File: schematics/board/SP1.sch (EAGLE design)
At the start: 12 parts

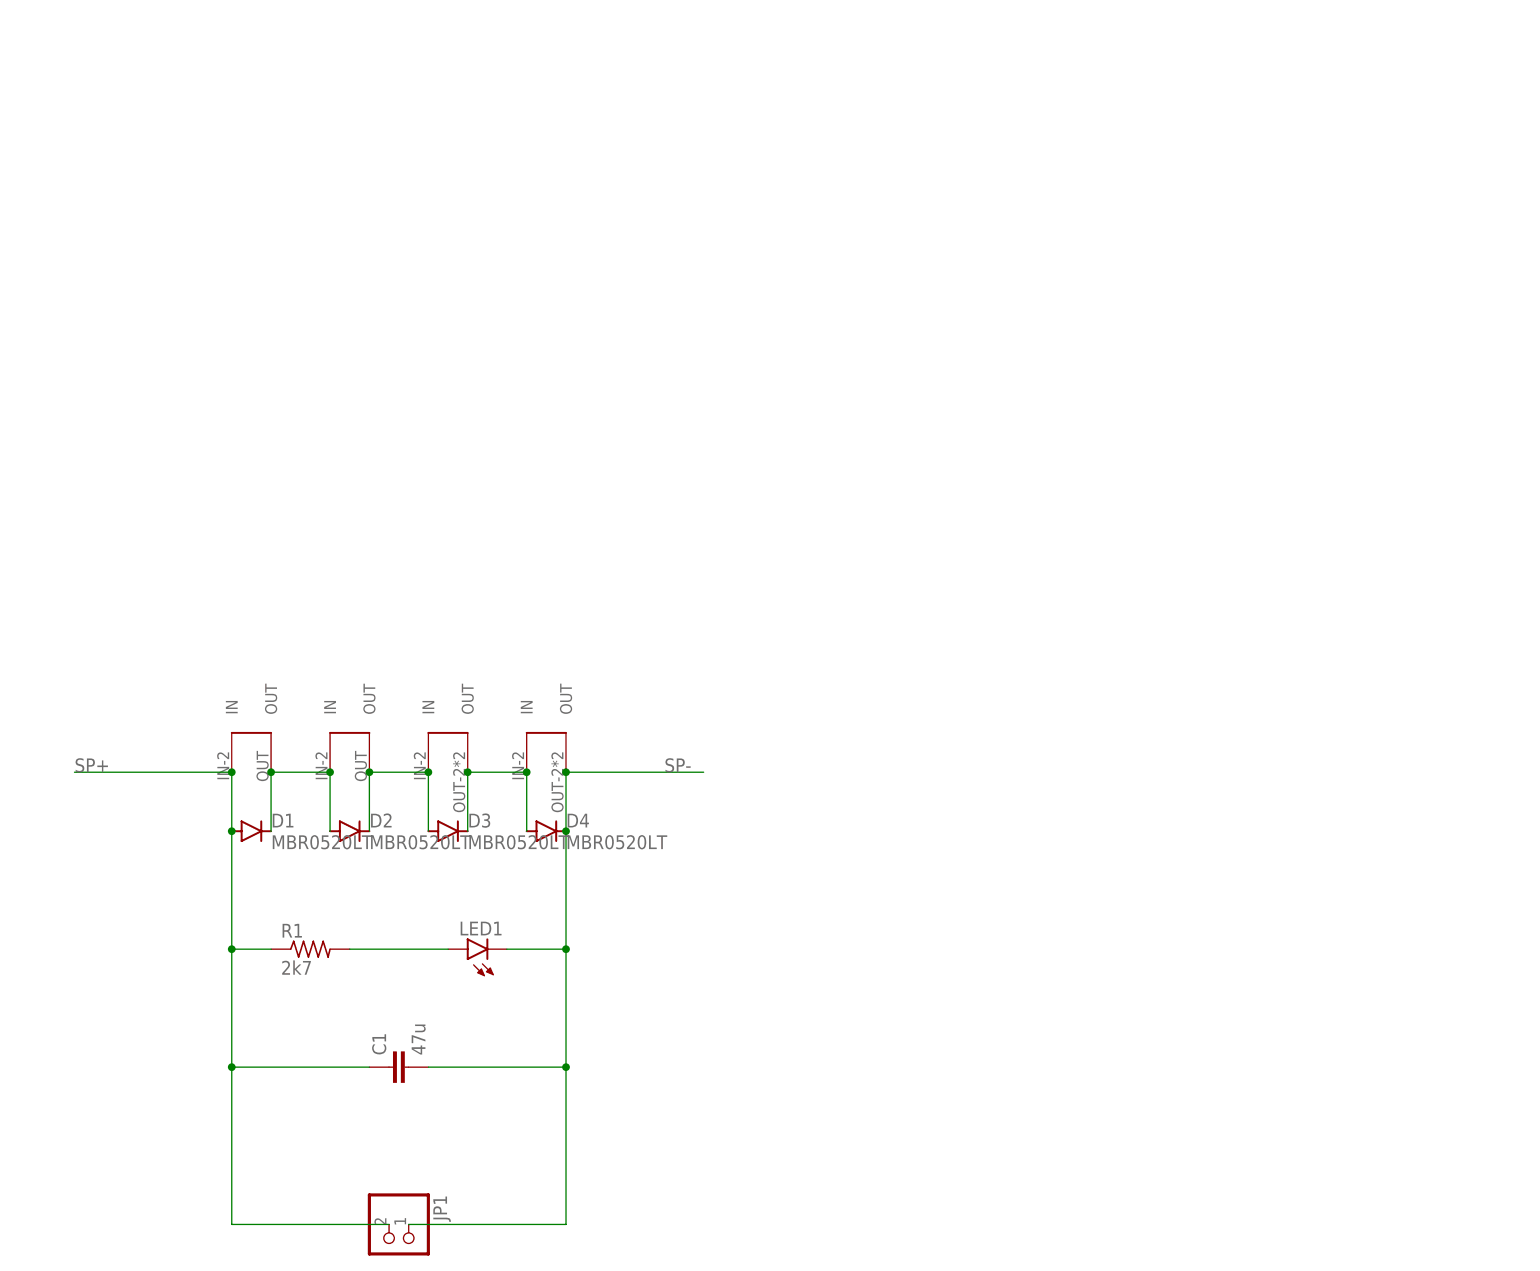
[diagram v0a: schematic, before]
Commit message: ПЛАТЫ, АААААААААААААААААААААААААААА
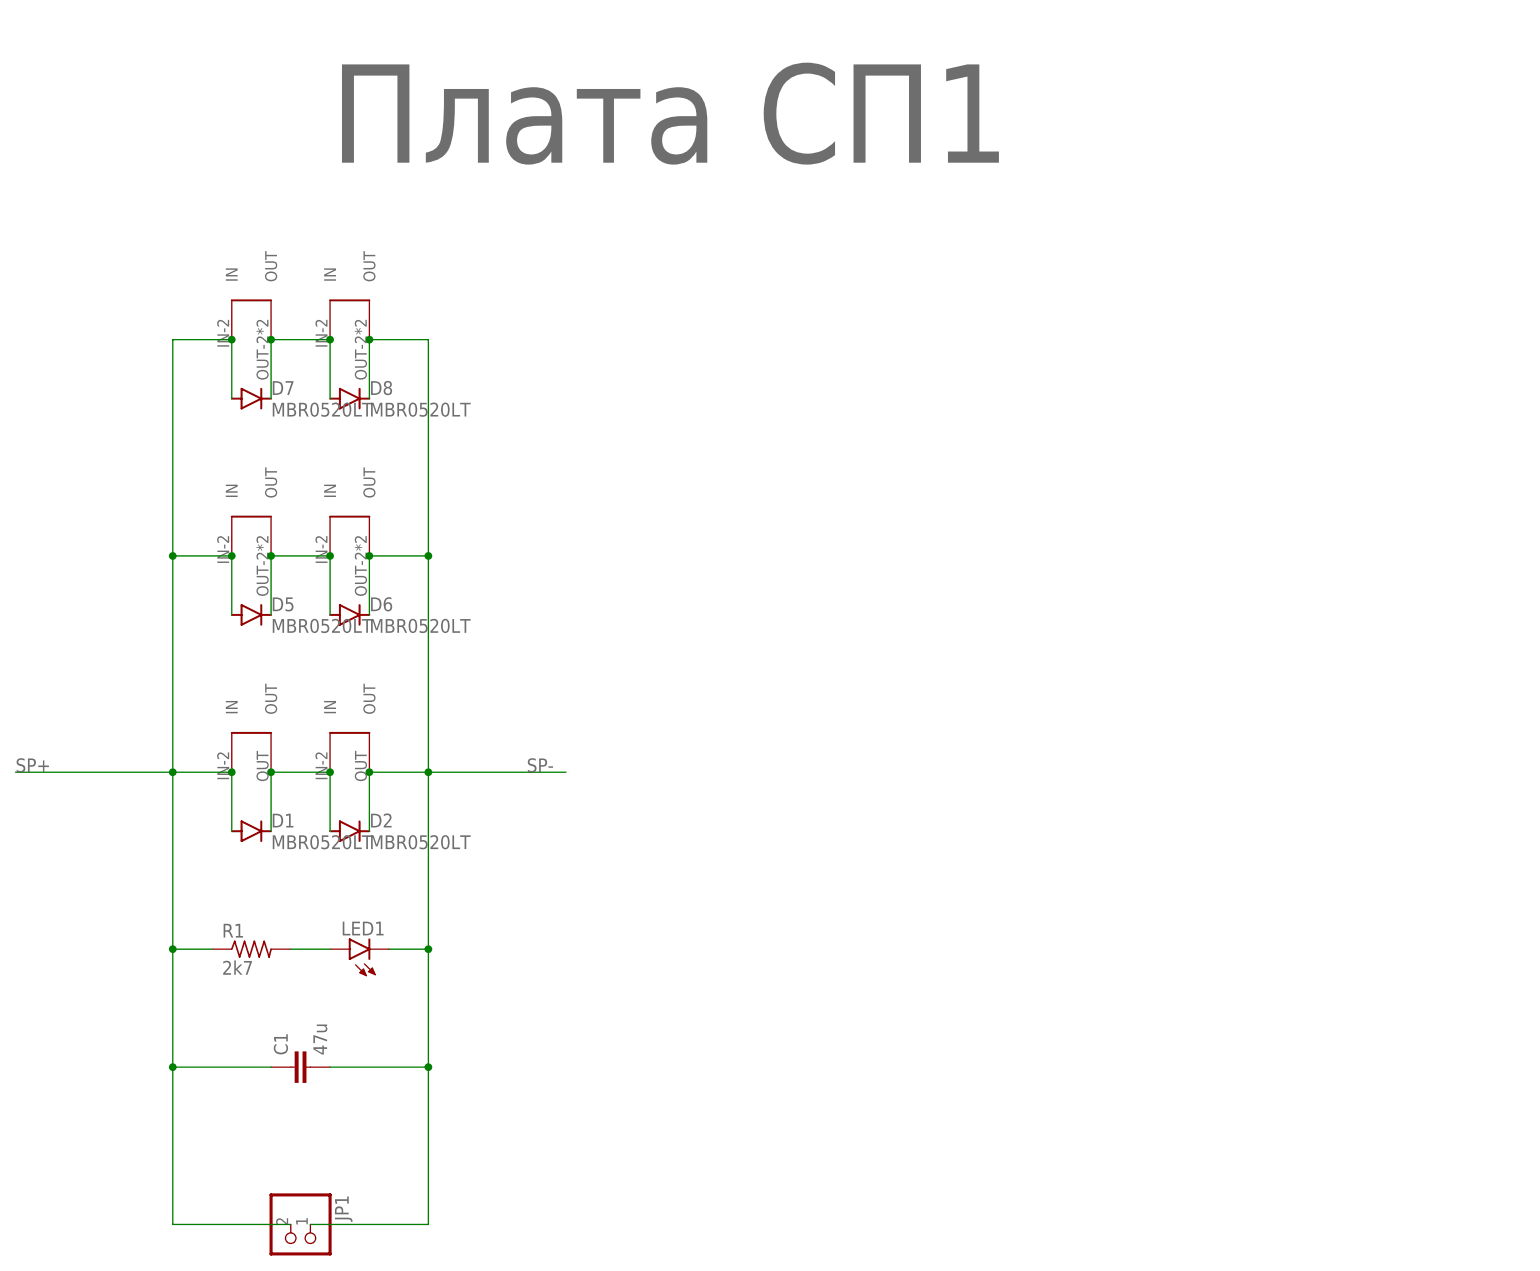
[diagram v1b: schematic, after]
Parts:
- removed D3, D4: MBR0520LT, diode:MBR0520LT
- removed U$4: SOLAR-2_0, CanCubeSat:SOLAR-2_0
- added D5, D6, D7, D8: MBR0520LT, diode:MBR0520LT
- added U$5, U$6, U$7, U$8: SOLAR-2_0, CanCubeSat:SOLAR-2_0
- U$3: value SOLAR-2_0 -> Плата СП1; device CanCubeSat:SOLAR-2_0 -> UNKNOWN-2024:LOGOPCB-""
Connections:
- removed net N$2: D2.C, D3.A, U$2.OUT, U$3.IN
- removed net N$3: D3.C, D4.A, U$3.OUT, U$4.IN
- new net N$6: D5.C, D6.A, U$5.OUT, U$6.IN
- new net N$8: D7.C, D8.A, U$7.OUT, U$8.IN
- net SP+: now also D5.A, D7.A, U$5.IN, U$7.IN
- net SP-: now also D2.C, D6.C, D8.C, U$2.OUT, U$6.OUT, U$8.OUT; no longer D4.C, U$4.OUT
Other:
- moved on the sheet: C1, JP1, LED1, R1
